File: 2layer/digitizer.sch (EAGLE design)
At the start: 23 parts, among them IC1 LT1763CS8-3

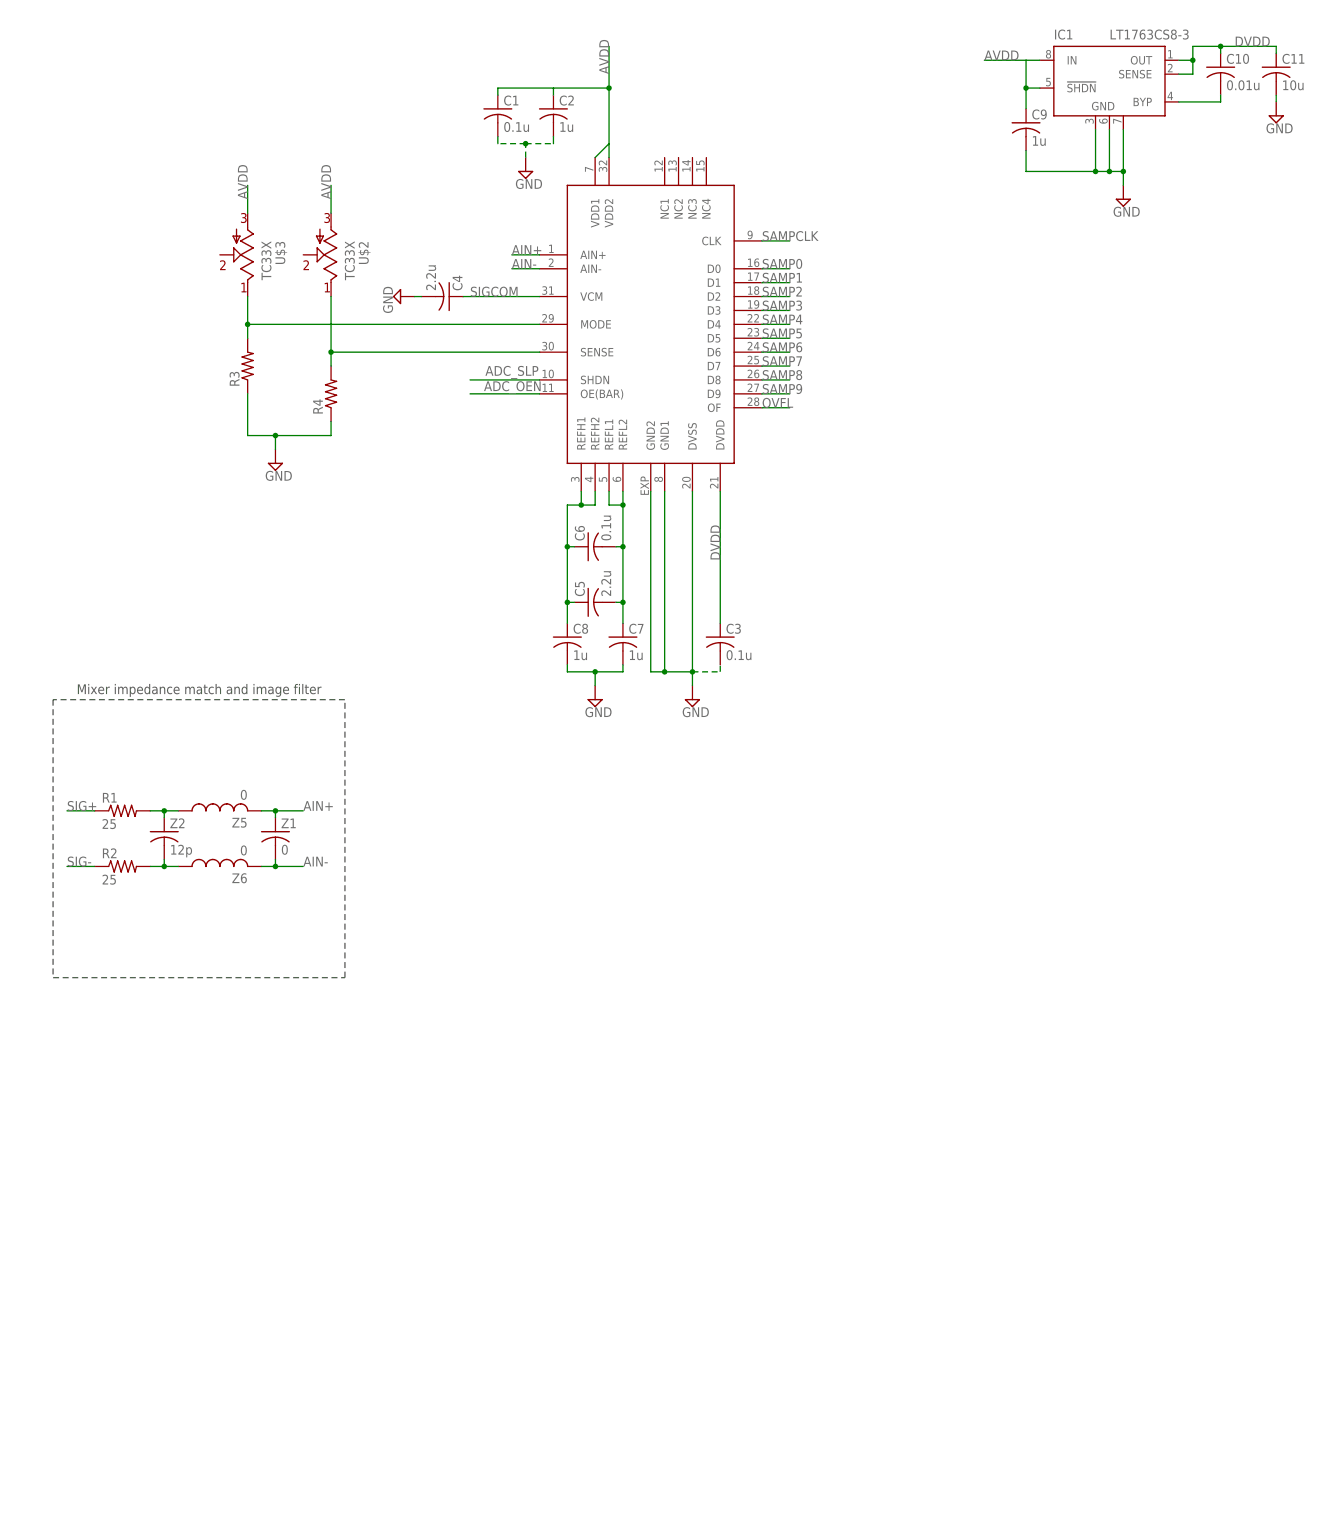
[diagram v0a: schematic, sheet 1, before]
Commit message: added some layout
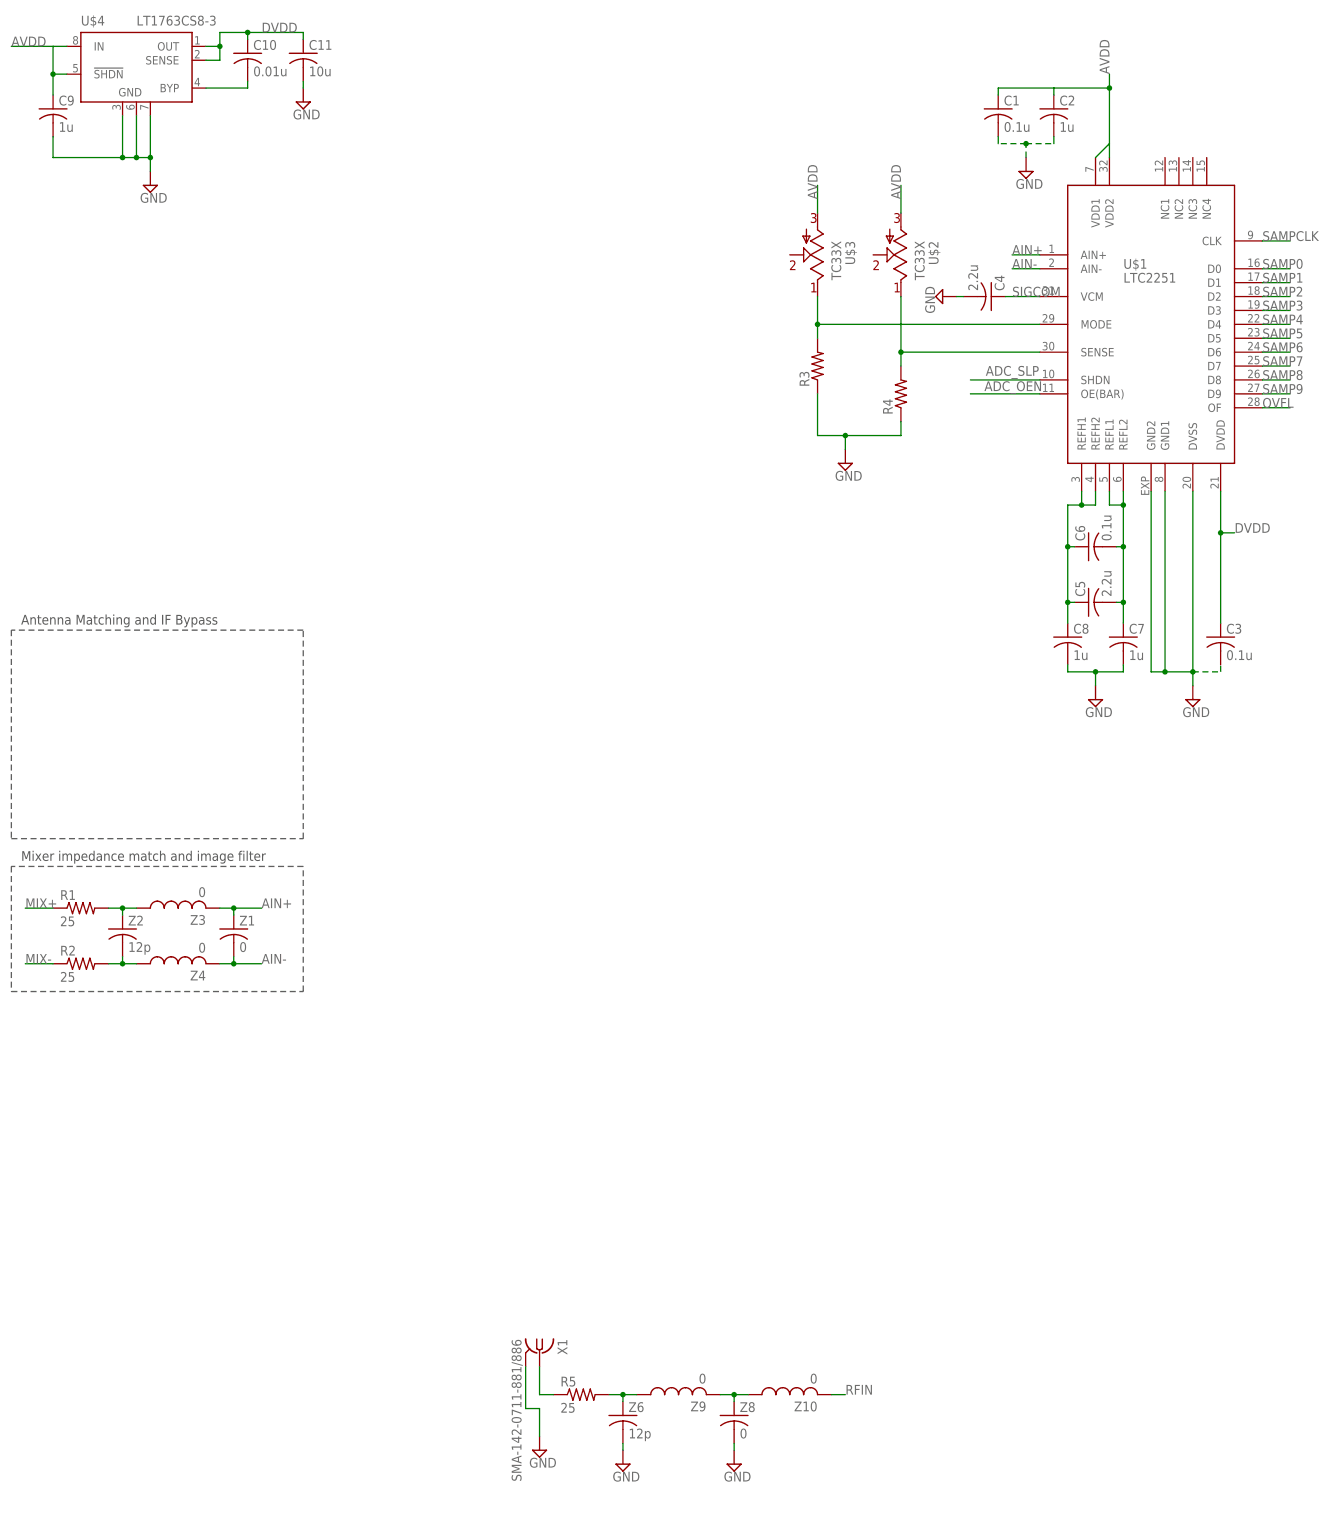
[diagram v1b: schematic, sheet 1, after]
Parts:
- removed IC1: LT1763CS8-3, linear-technology:LT1763CS8-3
- removed Z5: 0, components:L-US0805
- added R5: 25, resistor:R-US_R0402
- added U$4: LT1763CS8-3, linear-technology:LT1763CS8-3
- added X1: SMA-142-0711-881/886, con-coax:SMA-142-0711-881/886
- added Z10, Z3, Z4, Z9: 0, components:L-US0805
- added Z8: 0, resistor:C-USC0402
- Z6: value 0 -> 12p; device components:L-US0805 -> resistor:C-USC0402
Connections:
- net SIG+ renamed MIX+
- net SIG- renamed MIX-
- new net N$1: R5.2, Z6.1, Z9.1
- new net N$10: R5.1, X1.1
- new net RFILT: Z10.1, Z8.1, Z9.2
- new net RFIN: Z10.2
- net AIN+: now also Z3.2
- net AIN-: now also Z4.2
- net AVDD: now also U$4.!SHDN, U$4.IN; no longer IC1.!SHDN, IC1.IN
- net DVDD: now also U$4.OUT, U$4.SENSE; no longer IC1.OUT, IC1.SENSE
- net GND: now also U$4.GND@1, U$4.GND@2, U$4.GND@3, X1.2, Z6.2, Z8.2; no longer IC1.GND@1, IC1.GND@2, IC1.GND@3
- net N$6: now also Z3.1; no longer Z5.1
- net N$7: now also Z4.1; no longer Z6.1
- net N$9: now also U$4.BYP; no longer IC1.BYP
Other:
- note added: "Antenna Matching and IF Bypass"
- moved on the sheet: C1, C10, C11, C2, C3, C4, C5, C6, C7, C8, C9, R1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
